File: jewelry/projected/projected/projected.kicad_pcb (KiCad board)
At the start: 2 copper layers, 46 parts, among them J1 TOUCH, J3 DOCK, J4 Leds, J5 SWD, J6 EXT, Q1 BC847CL, U1 STM32L432KBU6, U2 MCP73812T-420I-OT, U3 PCA9306DCUR, U4 MCP1640BT-I/CHY‎, U5 TPS7A0533PDBVT, U6 LIS2DE12TR‎

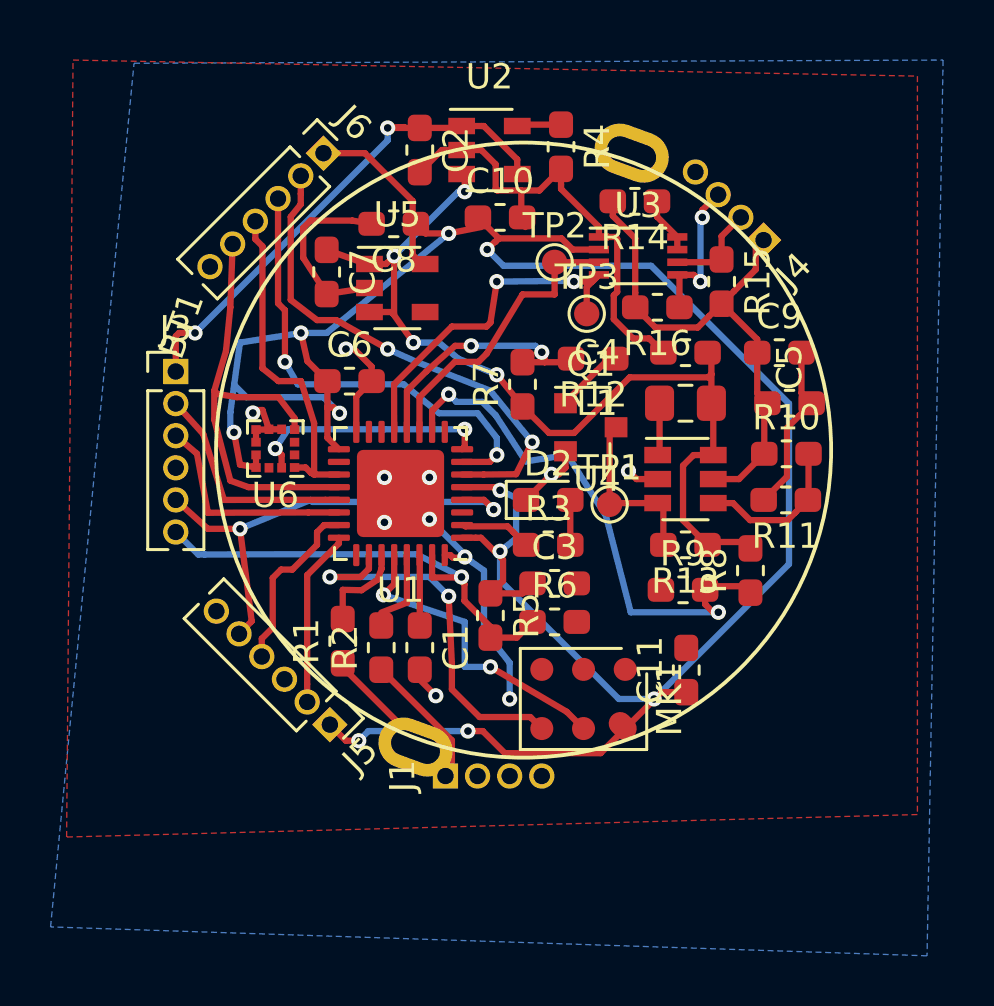
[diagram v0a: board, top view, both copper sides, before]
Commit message: projected: Routing almost complete
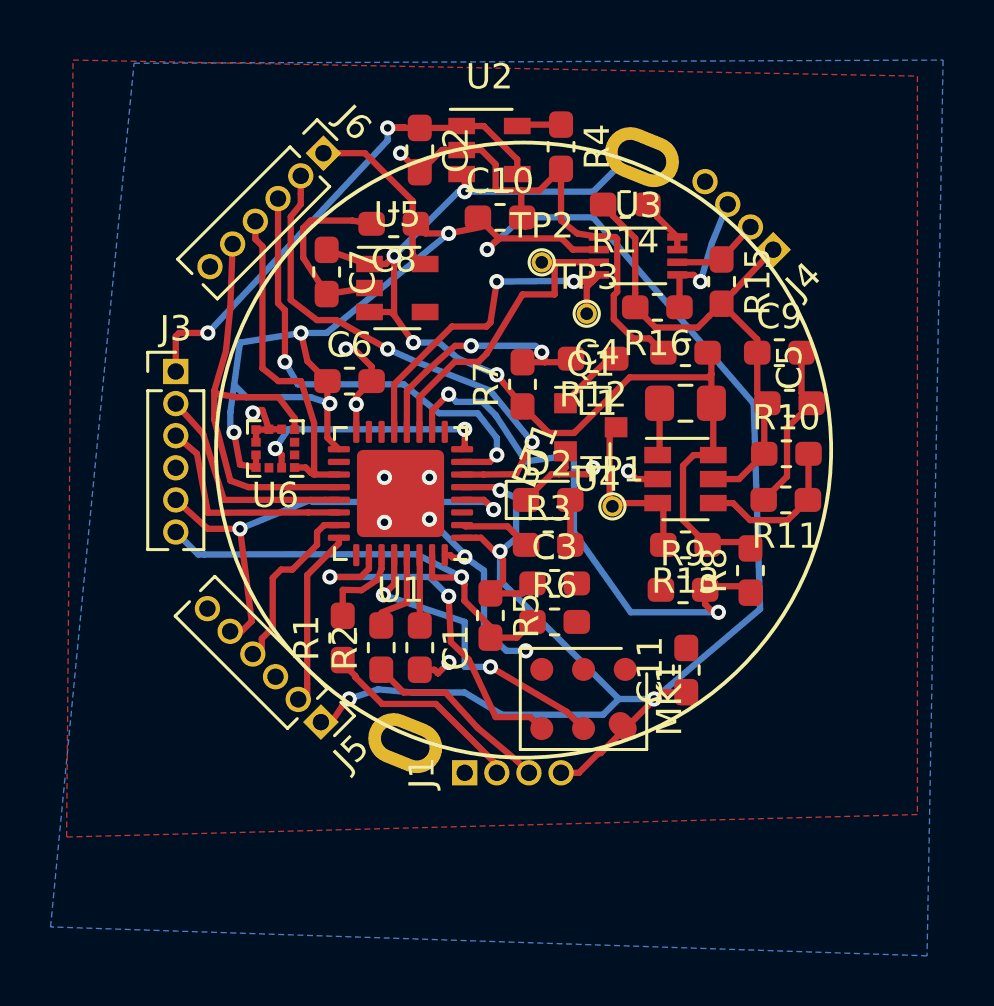
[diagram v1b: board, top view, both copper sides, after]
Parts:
- TP1, TP2, TP3: footprint TestPoint:TestPoint_Pad_D1.0mm -> projected:TestPoint_Mini
- moved J1 0.77 mm to (48.8, 63.1)
- moved J4 0.54 mm to (61.0, 42.4)
- moved TP2 0.51 mm to (51.8, 42.9)
- moved R14 0.40 mm to (55.1, 40.6)
- moved J5 0.37 mm to (43.1, 61.1)
- moved TP1 0.13 mm to (54.6, 52.6)
- moved R1 0.13 mm to (43.9, 57.8)
- turned BT1 to 68 degrees
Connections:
- J1 pad 1: Net-(J1-Pad1) -> GND
- J1 pad 3: GND -> Net-(J1-Pad3)
- R1 pad 1: Net-(J1-Pad1) -> Net-(J1-Pad2)
- R2 pad 1: Net-(J1-Pad2) -> Net-(J1-Pad3)
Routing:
- net Net-(J1-Pad3): track 0.00 -> 7.51 mm
- net +BATT: track 37.2 -> 44.4 mm
- net Net-(J1-Pad1): track 5.21 -> 0.00 mm
- net Net-(J1-Pad2): track 4.85 -> 8.26 mm
- net GND: track 47.3 -> 50.6 mm, vias 11 -> 13
- net VCC: track 105.6 -> 107.0 mm, vias 10 -> 9
- net /LED_DATA_5V: track 6.26 -> 5.59 mm, vias 2 -> 1
- net /SAI_SCK: track 15.1 -> 14.6 mm
- net /LED_CLK: track 11.8 -> 12.3 mm
